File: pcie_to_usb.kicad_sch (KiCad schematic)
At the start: 33 parts, among them J14 USB-A_Samtec_USB-A-S-F-B-VT_V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, J8 USB-A_Samtec_USB-A-S-F-B-VT_V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, U2 UPD720201K8-701-BAC-A, U3 AP22615A_TSOT26, U4 AP22615A_TSOT26

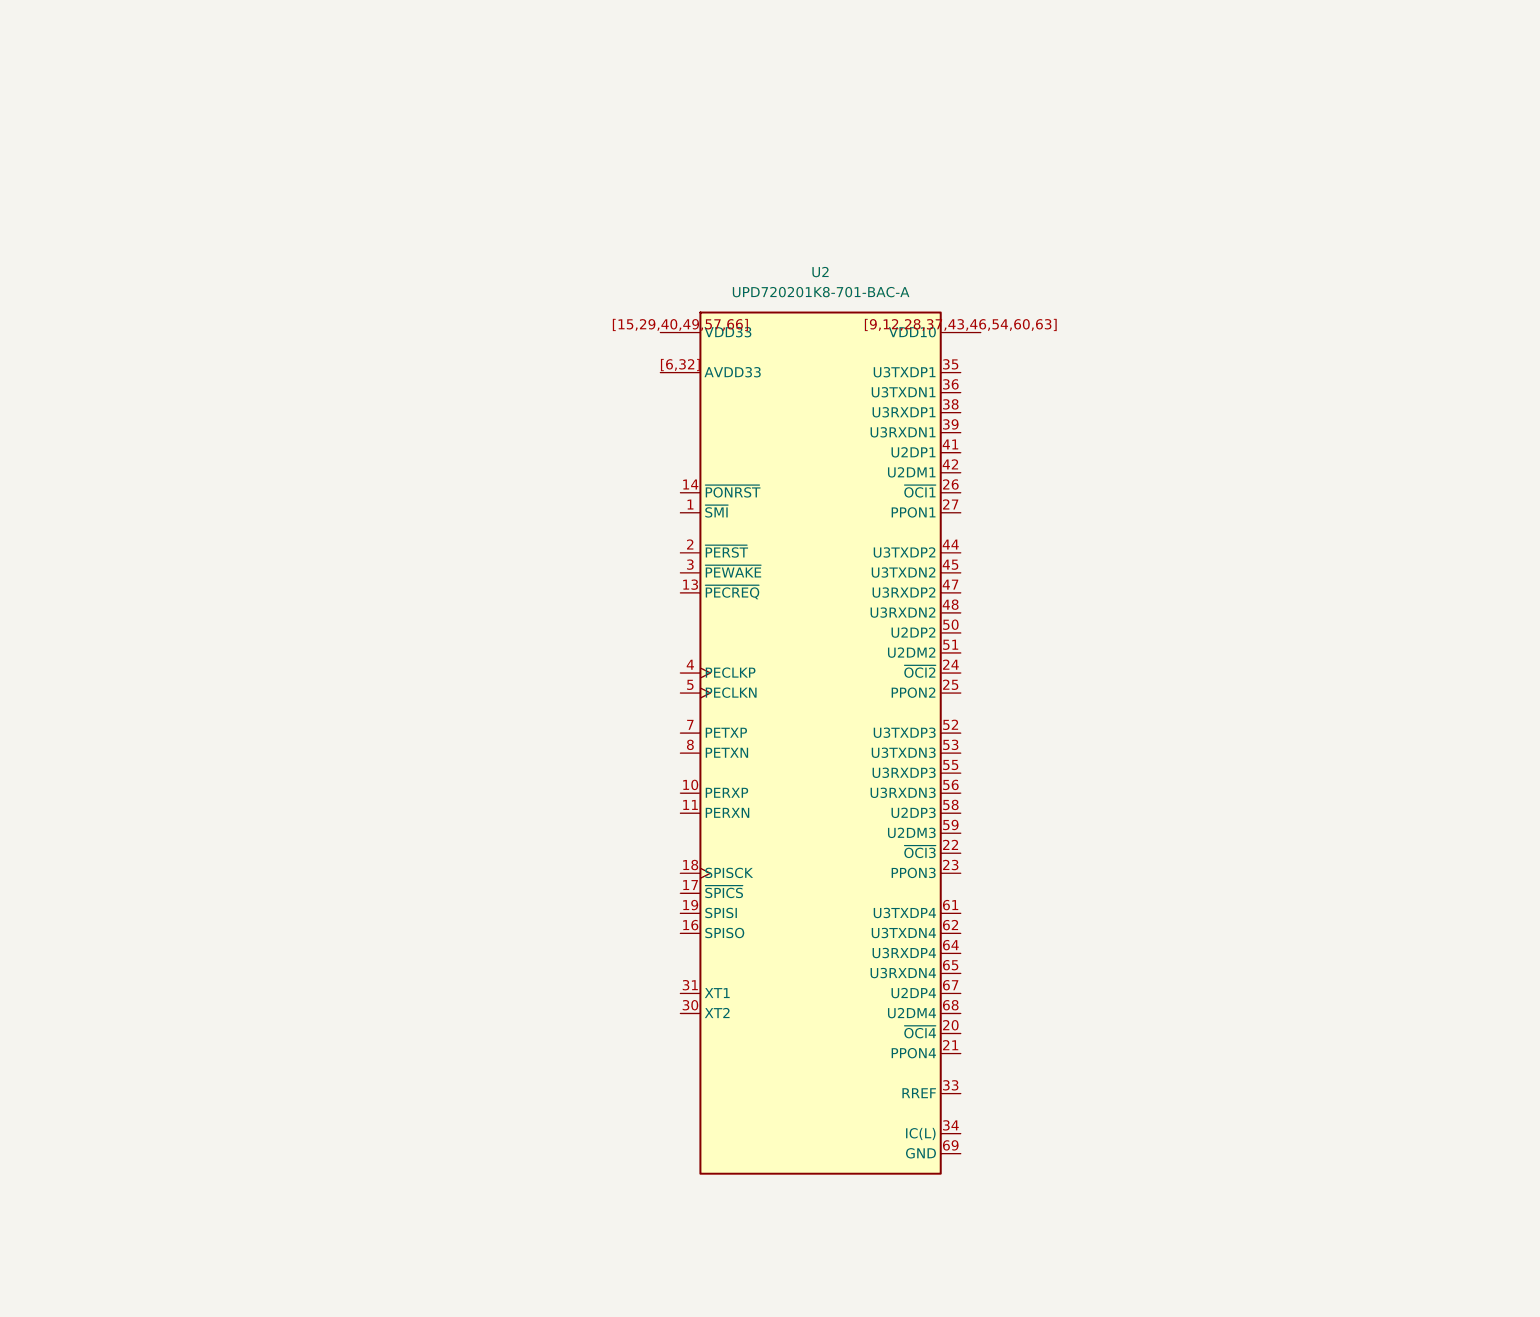
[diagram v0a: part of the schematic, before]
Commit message: [#100720] Start USB section
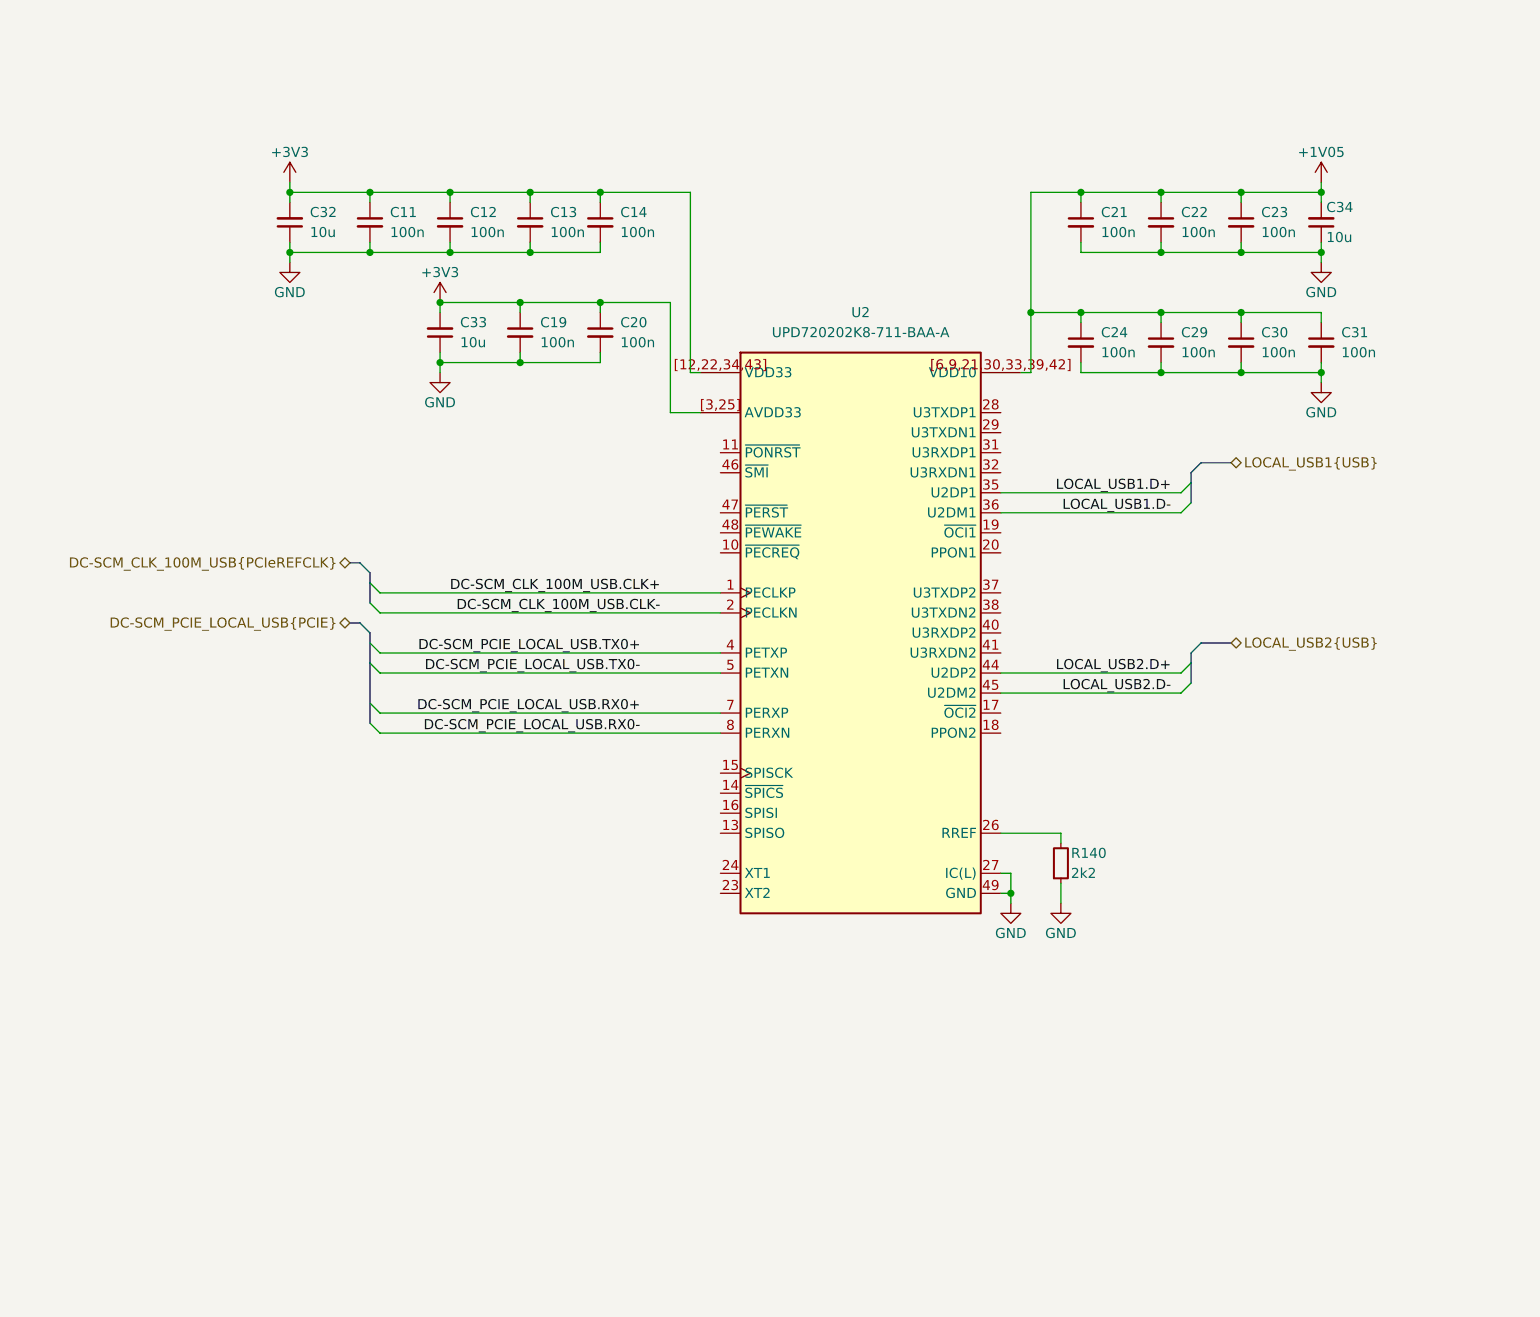
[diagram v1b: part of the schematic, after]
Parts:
- removed U2: UPD720201K8-701-BAC-A, antmicro-footprints:QFN-68-1EP_8x8mm_P0.4mm, symbol antmicroInterfaceControllers:UPD720201K8-701-BAC-A
- added C11, C12, C13, C14, C19, C20, C21, C22, C23, C24, C29, C30, C31: C_100n_0402, antmicro-footprints:C_0402_1005Metric, symbol antmicroCapacitors0402:C_100n_0402
- added C32, C33, C34: C_10u_10V_0402, antmicro-footprints:C_0402_1005Metric, symbol antmicroCapacitors0402:C_10u_10V_0402
- added R140: R_2k2_0402, antmicro-footprints:R_0402_1005Metric, symbol antmicroResistors0402:R_2k2_0402
- added U2: UPD720202K8-711-BAA-A, antmicro-footprints:QFN-48-1EP_7x7mm, symbol antmicroInterfaceControllers:UPD720202K8-711-BAA-A
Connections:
- net GND: now also C11.2, C12.2, C13.2, C14.2, C19.2, C20.2, C21.2, C22.2, C23.2, C24.2, C29.2, C30.2, C31.2, C32.1, C33.1, C34.1, R140.1, U2.27 (IC(L)), U2.49 (GND)
- net LOCAL_USB1.D+: now also U2.35 (U2DP1)
- net LOCAL_USB1.D-: now also U2.36 (U2DM1)
- net LOCAL_USB2.D+: now also U2.44 (U2DP2)
- net LOCAL_USB2.D-: now also U2.45 (U2DM2)
- new net: R140.2, U2.26 (RREF)
- new net +1V05: C21.1, C22.1, C23.1, C24.1, C29.1, C30.1, C31.1, C34.2, U2.[6,9,21,30,33,39,42] (VDD10)
- new net +3V3: C11.1, C12.1, C13.1, C14.1, C19.1, C20.1, C32.2, C33.2, U2.[12,22,34,43] (VDD33), U2.[3,25] (AVDD33)
- new net DC-SCM_CLK_100M_USB.CLK+: U2.1 (PECLKP)
- new net DC-SCM_CLK_100M_USB.CLK-: U2.2 (PECLKN)
- new net DC-SCM_PCIE_LOCAL_USB.RX0+: U2.7 (PERXP)
- new net DC-SCM_PCIE_LOCAL_USB.RX0-: U2.8 (PERXN)
- new net DC-SCM_PCIE_LOCAL_USB.TX0+: U2.4 (PETXP)
- new net DC-SCM_PCIE_LOCAL_USB.TX0-: U2.5 (PETXN)
